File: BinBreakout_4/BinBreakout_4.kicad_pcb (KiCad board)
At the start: 2 copper layers, 55 x 19 mm, 7 parts

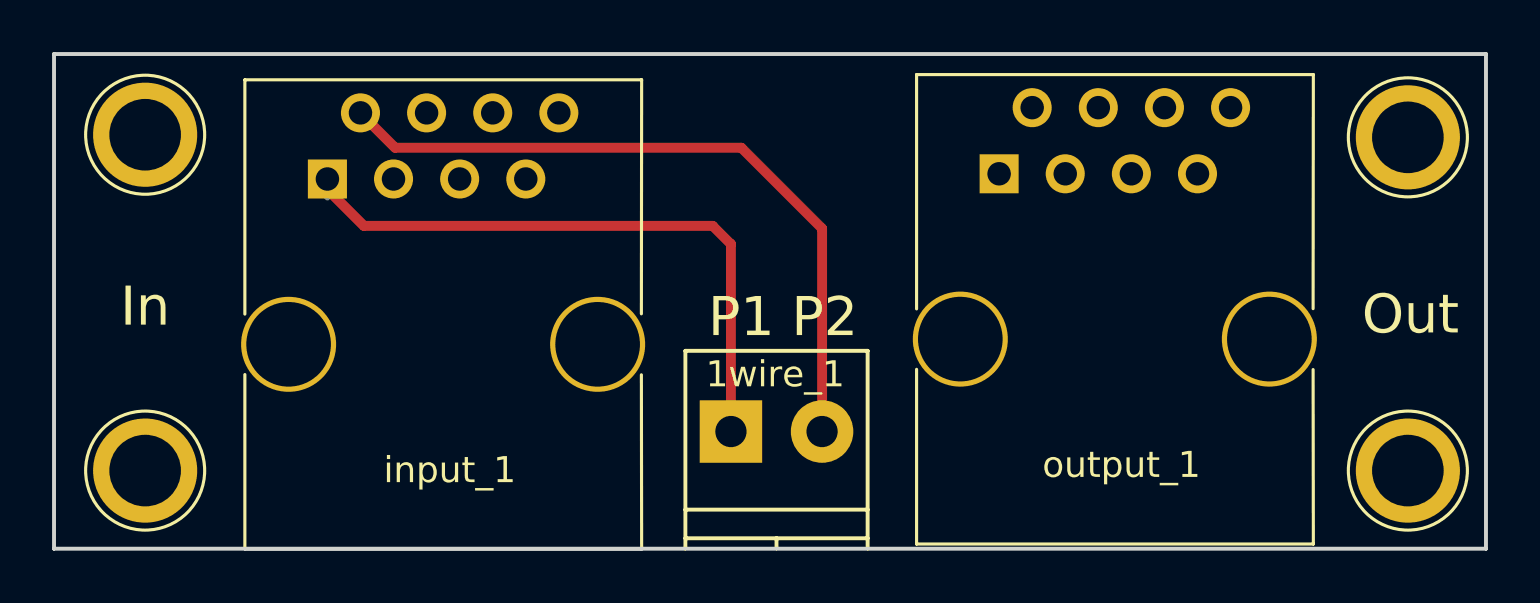
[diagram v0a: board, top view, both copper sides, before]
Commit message: version 1 of the boards. getting printed PCBs from OSH park
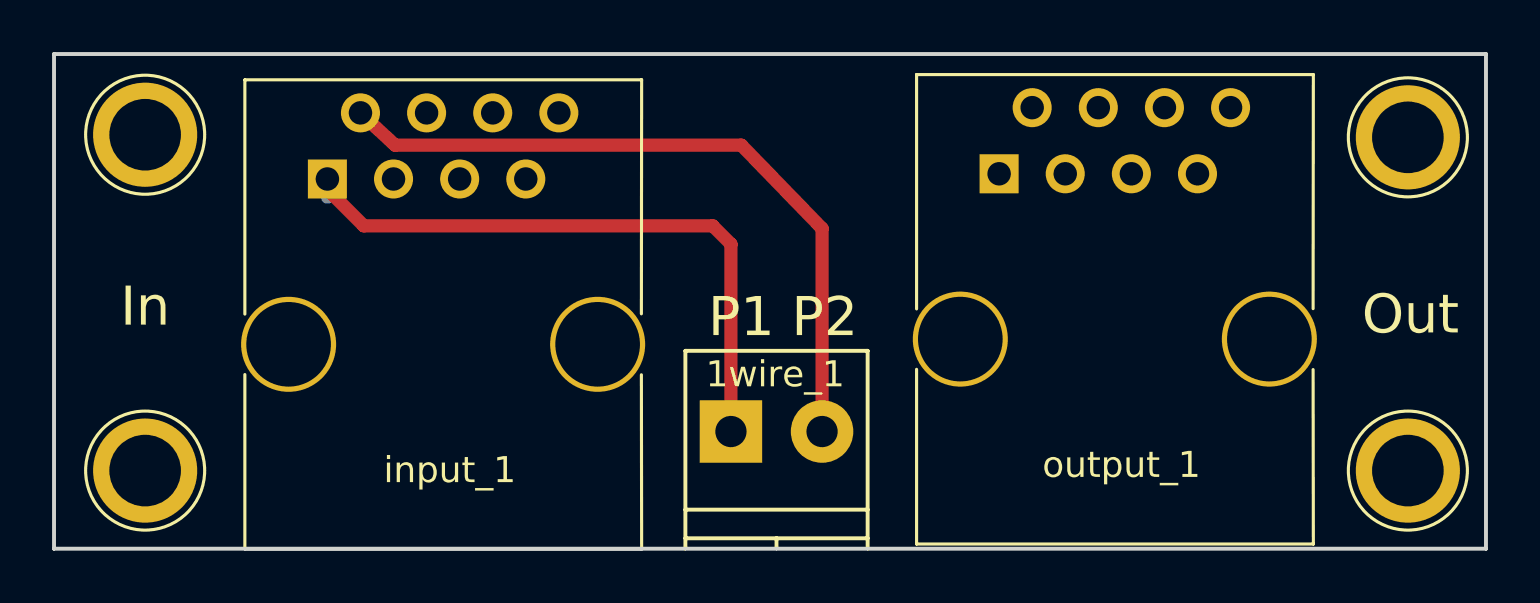
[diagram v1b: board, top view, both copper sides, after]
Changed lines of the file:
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@@
     (links 2)
     (no_connects 0)
-    (area 100.924999 75.924999 156.075001 95.075001)
+    (area 100.924999 75.1246 156.075001 97.5274)
     (thickness 1.6002)
     (drawings 8)
@@
   )
   (setup
-    (last_trace_width 0.1524)
+    (last_trace_width 0.508)
     (user_trace_width 0.1524)
     (user_trace_width 0.254)
@@
     (user_via 0.6858 0.3302)
     (user_via 0.6858 0.4)
+    (user_via 0.762 0.4572)
     (user_via 1.905 0.3302)
     (uvia_size 0.762)
@@
   (gr_line (start 156 76) (end 156 95) (angle 90) (layer Edge.Cuts) (width 0.15))
   (gr_line (start 156 95) (end 101 95) (angle 90) (layer Edge.Cuts) (width 0.15))
-  (segment (start 111.5 80.8) (end 111.5 81.2) (width 0.381) (layer Top) (net 1))
-  (segment (start 111.5 81.2) (end 112.9 82.6) (width 0.381) (layer Top) (net 1))
-  (segment (start 127 83.3) (end 127 90.5) (width 0.381) (layer Top) (net 1))
-  (segment (start 126.3 82.6) (end 127 83.3) (width 0.381) (layer Top) (net 1))
-  (segment (start 112.9 82.6) (end 126.3 82.6) (width 0.381) (layer Top) (net 1))
-  (segment (start 111.5 80.8) (end 111.5 81.5) (width 0.254) (layer Bottom) (net 1))
-  (segment (start 112.77 78.26) (end 112.77 78.27) (width 0.381) (layer Top) (net 2))
-  (segment (start 112.77 78.27) (end 114.1 79.6) (width 0.381) (layer Top) (net 2))
-  (segment (start 130.5 82.7) (end 130.5 90.5) (width 0.381) (layer Top) (net 2))
-  (segment (start 127.4 79.6) (end 130.5 82.7) (width 0.381) (layer Top) (net 2))
-  (segment (start 114.1 79.6) (end 127.4 79.6) (width 0.381) (layer Top) (net 2))
-  (segment (start 112.77 78.26) (end 112.77 78.23) (width 0.254) (layer Bottom) (net 2))
-  (segment (start 112.77 78.26) (end 112.86 78.26) (width 0.254) (layer Bottom) (net 2))
+  (segment (start 111.5 80.8) (end 111.5 81.2) (width 0.508) (layer Top) (net 1))
+  (segment (start 111.5 81.2) (end 112.9 82.6) (width 0.508) (layer Top) (net 1))
+  (segment (start 127 83.3) (end 127 90.5) (width 0.508) (layer Top) (net 1))
+  (segment (start 126.3 82.6) (end 127 83.3) (width 0.508) (layer Top) (net 1))
+  (segment (start 112.9 82.6) (end 126.3 82.6) (width 0.508) (layer Top) (net 1))
+  (segment (start 111.5 80.8) (end 111.5 81.5) (width 0.508) (layer Bottom) (net 1))
+  (segment (start 112.77 78.26) (end 112.77 78.27) (width 0.508) (layer Top) (net 2))
+  (segment (start 112.77 78.27) (end 114.1 79.5) (width 0.508) (layer Top) (net 2))
+  (segment (start 130.5 82.7) (end 130.5 90.5) (width 0.508) (layer Top) (net 2))
+  (segment (start 127.4 79.5) (end 130.5 82.7) (width 0.508) (layer Top) (net 2))
+  (segment (start 114.1 79.5) (end 127.4 79.5) (width 0.508) (layer Top) (net 2))
+  (segment (start 112.77 78.26) (end 112.77 78.23) (width 0.508) (layer Bottom) (net 2))
+  (segment (start 112.77 78.26) (end 112.86 78.26) (width 0.508) (layer Bottom) (net 2))
   (segment (start 116.58 80.8) (end 116.58 80.98) (width 0.381) (layer Top) (net 5))
   (segment (start 116.58 80.8) (end 116.58 81.28) (width 0.254) (layer Bottom) (net 5))
